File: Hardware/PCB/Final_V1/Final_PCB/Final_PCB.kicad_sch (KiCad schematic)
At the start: 0 parts

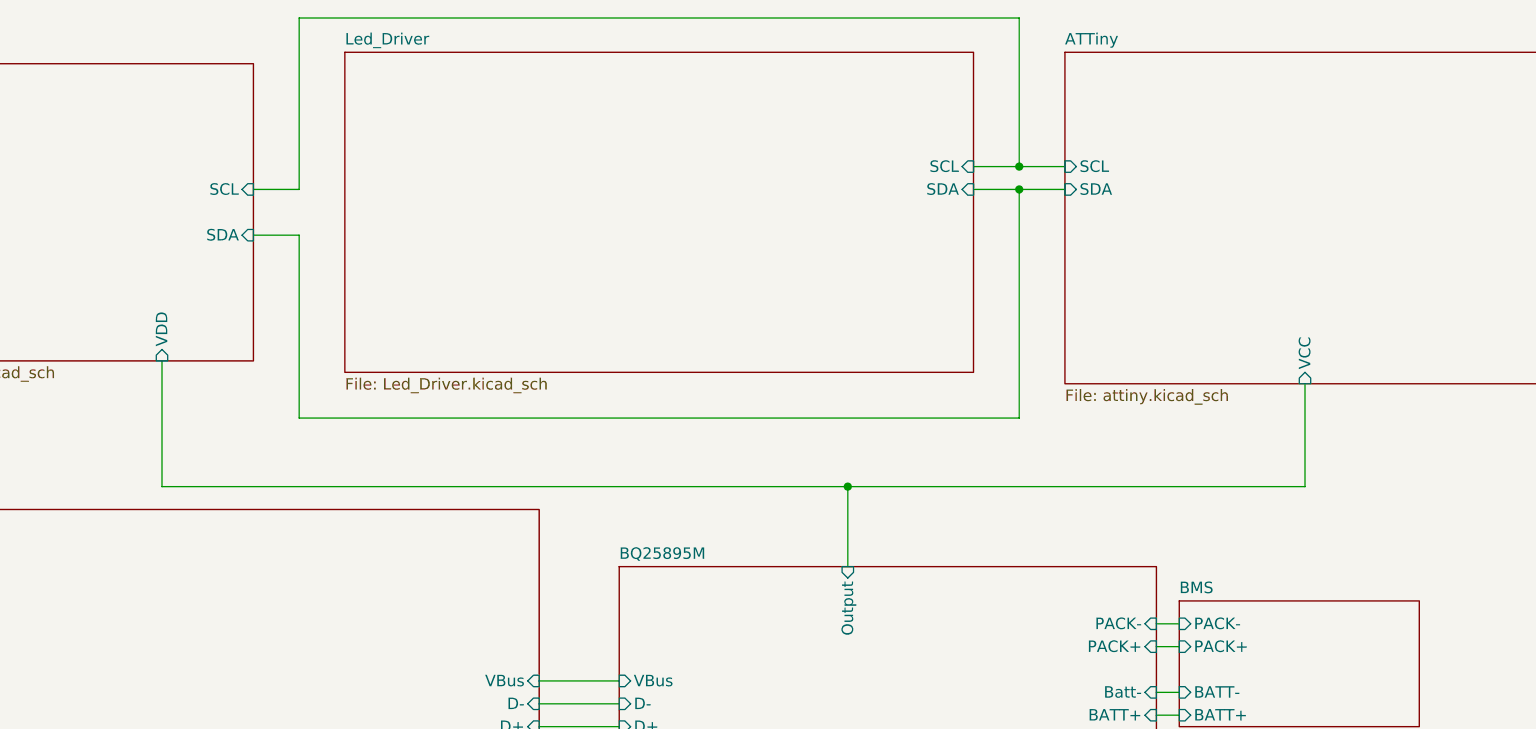
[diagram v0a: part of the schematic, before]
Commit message: fixed Schematics
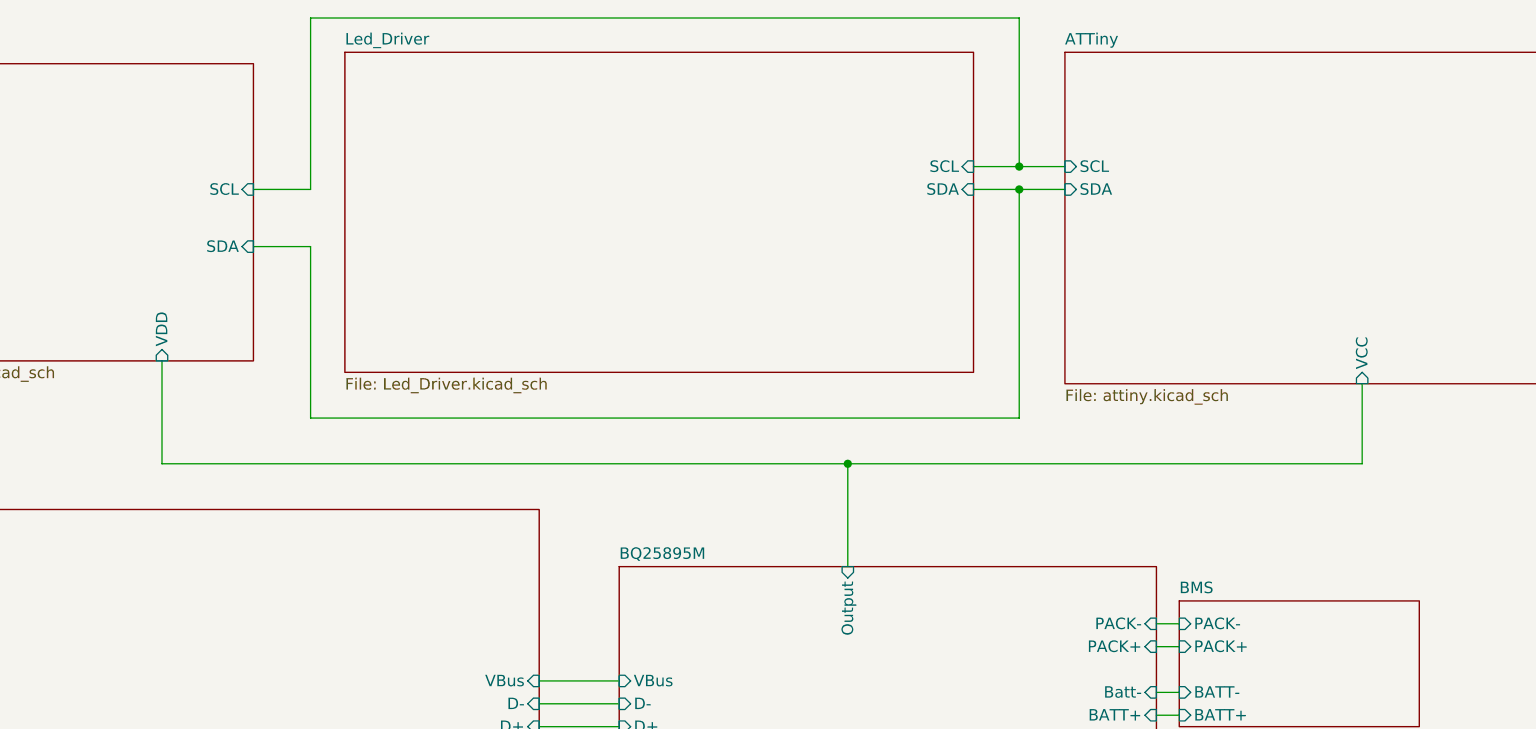
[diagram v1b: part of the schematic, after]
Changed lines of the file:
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@@
 	(paper "A4")
+	(junction
+		(at 121.92 67.31)
+		(diameter 0)
+		(color 0 0 0 0)
+	)
 	(junction
 		(at 140.97 36.83)
@@
 	)
 	(junction
-		(at 121.92 69.85)
-		(diameter 0)
-		(color 0 0 0 0)
-	)
-	(junction
 		(at 140.97 34.29)
 		(diameter 0)
@@
 	(wire
 		(pts
-			(xy 55.88 41.91) (xy 60.96 41.91)
-		)
-		(stroke
-			(width 0)
-			(type default)
-		)
-	)
-	(wire
-		(pts
-			(xy 60.96 41.91) (xy 60.96 62.23)
+			(xy 55.88 43.18) (xy 62.23 43.18)
+		)
+		(stroke
+			(width 0)
+			(type default)
+		)
+	)
+	(wire
+		(pts
+			(xy 62.23 43.18) (xy 62.23 62.23)
 		)
 		(stroke
@@
 	(wire
 		(pts
-			(xy 121.92 69.85) (xy 121.92 78.74)
+			(xy 121.92 67.31) (xy 121.92 78.74)
+		)
+		(stroke
+			(width 0)
+			(type default)
+		)
+	)
+	(wire
+		(pts
+			(xy 45.72 67.31) (xy 121.92 67.31)
 		)
 		(stroke
@@
 	(wire
 		(pts
-			(xy 45.72 55.88) (xy 45.72 69.85)
-		)
-		(stroke
-			(width 0)
-			(type default)
-		)
-	)
-	(wire
-		(pts
 			(xy 87.63 93.98) (xy 96.52 93.98)
 		)
@@
 	(wire
 		(pts
+			(xy 45.72 67.31) (xy 45.72 55.88)
+		)
+		(stroke
+			(width 0)
+			(type default)
+		)
+	)
+	(wire
+		(pts
 			(xy 87.63 91.44) (xy 96.52 91.44)
 		)
@@
 	(wire
 		(pts
-			(xy 172.72 58.42) (xy 172.72 69.85)
-		)
-		(stroke
-			(width 0)
-			(type default)
-		)
-	)
-	(wire
-		(pts
-			(xy 172.72 69.85) (xy 121.92 69.85)
-		)
-		(stroke
-			(width 0)
-			(type default)
-		)
-	)
-	(wire
-		(pts
-			(xy 60.96 36.83) (xy 60.96 17.78)
-		)
-		(stroke
-			(width 0)
-			(type default)
-		)
-	)
-	(wire
-		(pts
-			(xy 60.96 17.78) (xy 140.97 17.78)
-		)
-		(stroke
-			(width 0)
-			(type default)
-		)
-	)
-	(wire
-		(pts
-			(xy 45.72 69.85) (xy 121.92 69.85)
+			(xy 121.92 67.31) (xy 179.07 67.31)
+		)
+		(stroke
+			(width 0)
+			(type default)
+		)
+	)
+	(wire
+		(pts
+			(xy 62.23 36.83) (xy 62.23 17.78)
+		)
+		(stroke
+			(width 0)
+			(type default)
+		)
+	)
+	(wire
+		(pts
+			(xy 62.23 17.78) (xy 140.97 17.78)
 		)
 		(stroke
@@
 	(wire
 		(pts
-			(xy 60.96 62.23) (xy 140.97 62.23)
+			(xy 62.23 62.23) (xy 140.97 62.23)
 		)
 		(stroke
@@
 	(wire
 		(pts
+			(xy 179.07 67.31) (xy 179.07 58.42)
+		)
+		(stroke
+			(width 0)
+			(type default)
+		)
+	)
+	(wire
+		(pts
 			(xy 156.21 95.25) (xy 158.75 95.25)
 		)
@@
 	(wire
 		(pts
-			(xy 55.88 36.83) (xy 60.96 36.83)
+			(xy 55.88 36.83) (xy 62.23 36.83)
 		)
 		(stroke
@@
 		)
 		(pin "VCC" input
-			(at 172.72 58.42 270)
+			(at 179.07 58.42 270)
 			(effects
 				(font
@@
 		)
 		(pin "SDA" input
-			(at 55.88 41.91 0)
-			(effects
-				(font
+			(at 55.88 43.18 0)
+			(effects
+				(font

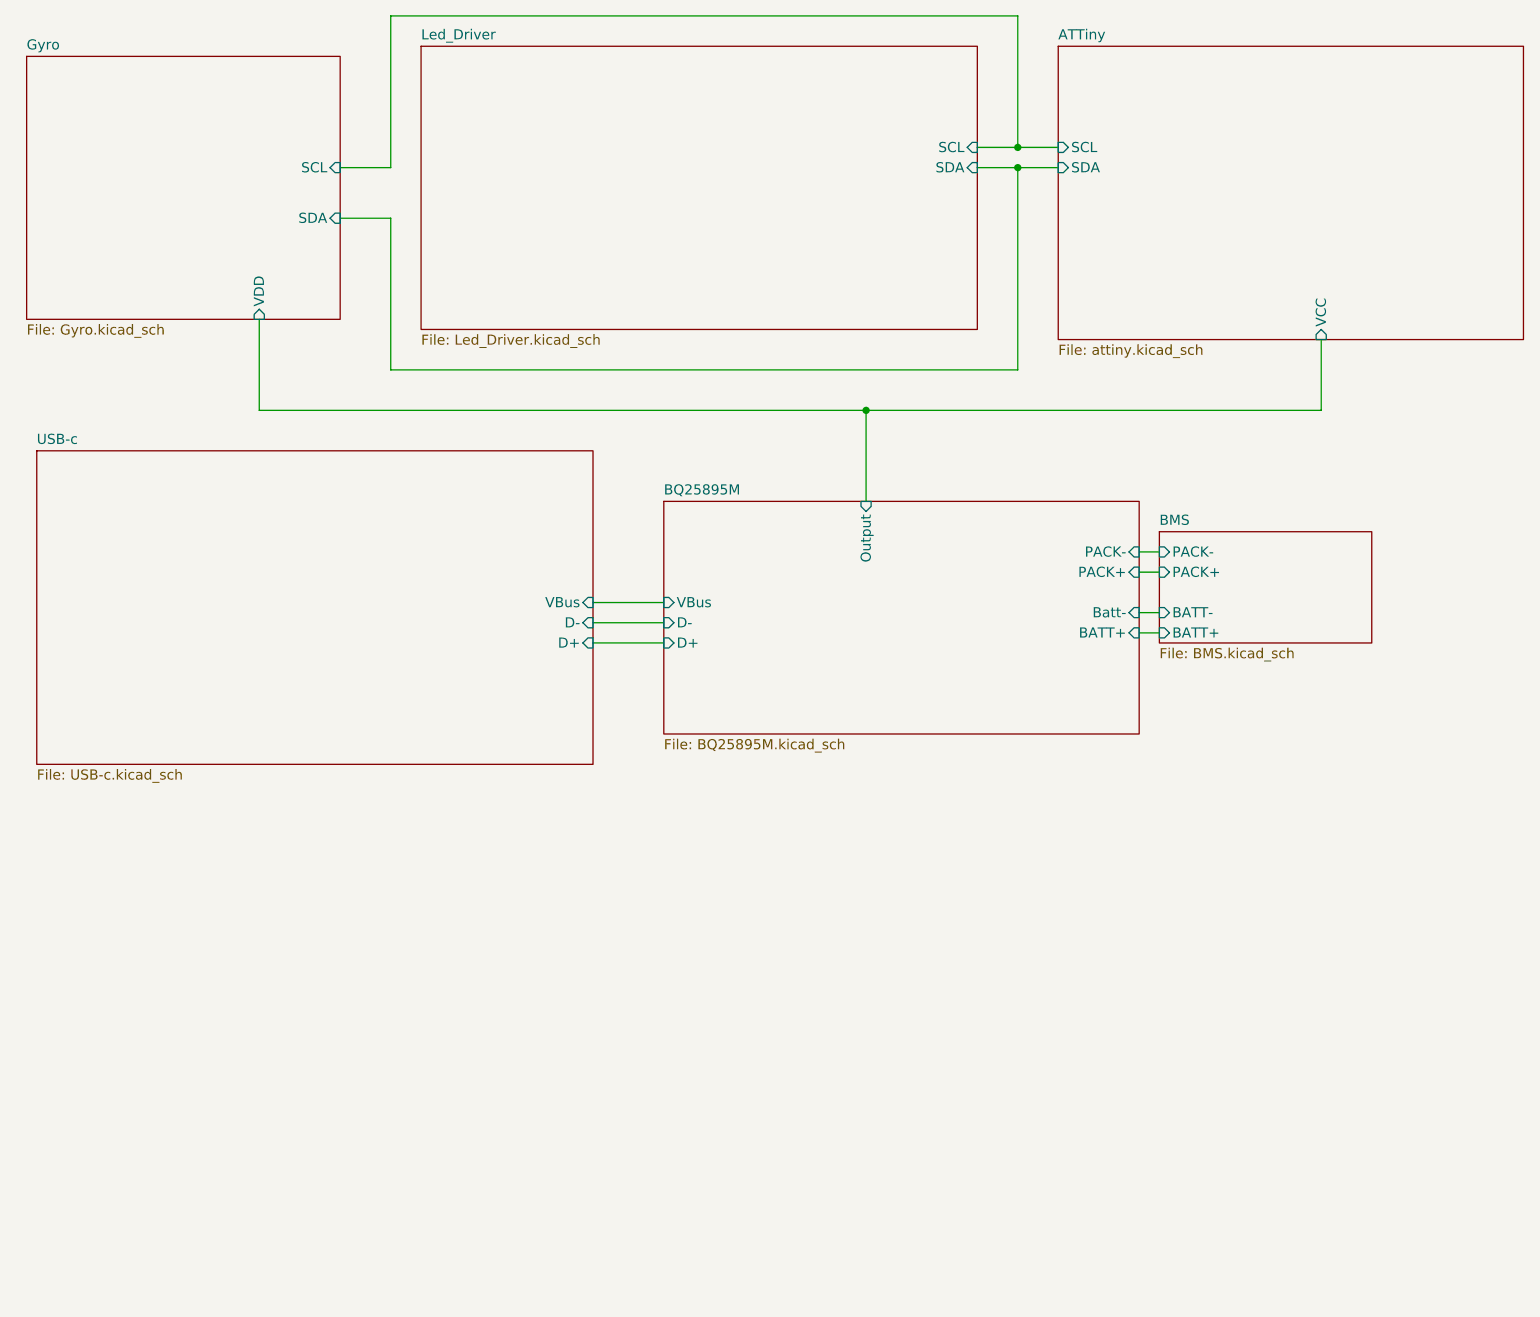
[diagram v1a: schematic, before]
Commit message: fixed last commit, because it was wrong
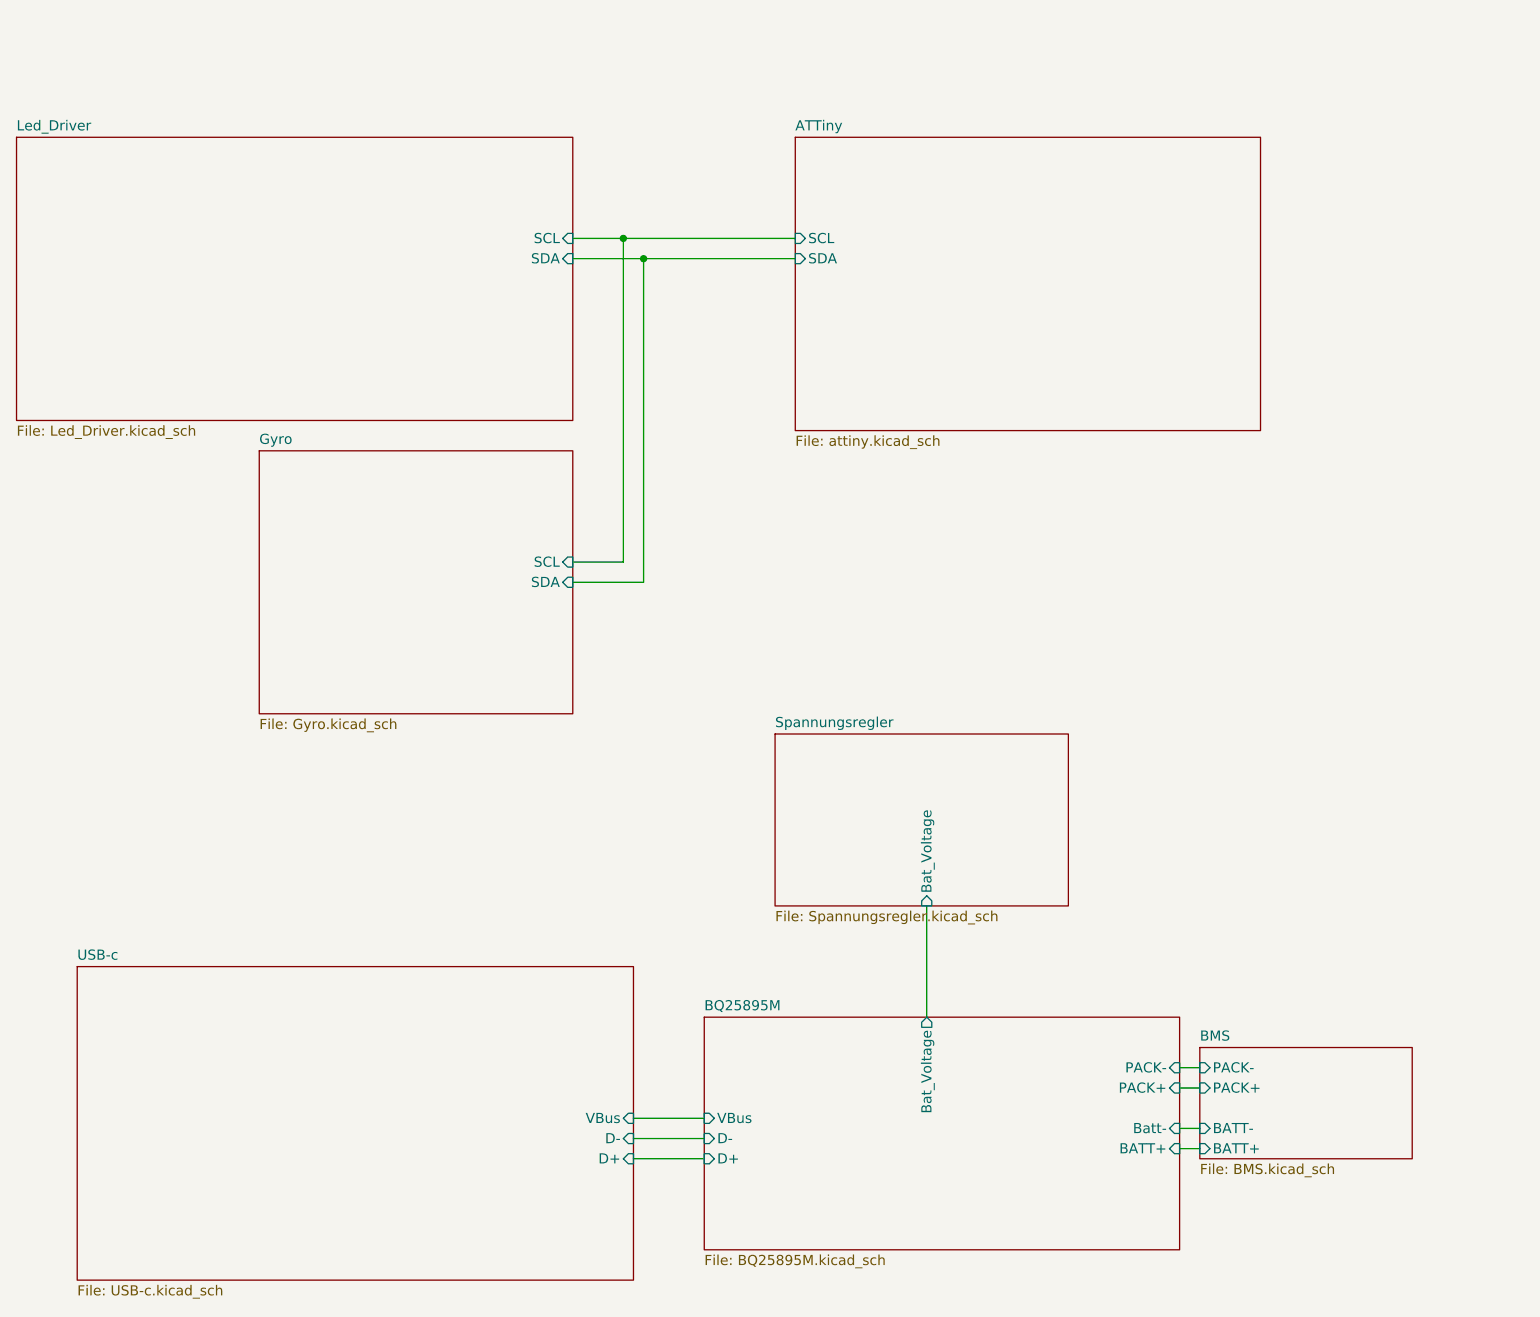
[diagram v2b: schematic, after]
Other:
- added sheet Spannungsregler (Spannungsregler.kicad_sch)
- sheet ATTiny ports: added none; removed VCC
- sheet BQ25895M ports: added Bat_Voltage; removed Output
- sheet Gyro ports: added none; removed VDD
